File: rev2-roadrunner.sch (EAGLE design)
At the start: 22 parts, among them J1 USB_MINI-B_SMT, Y1 16MHz

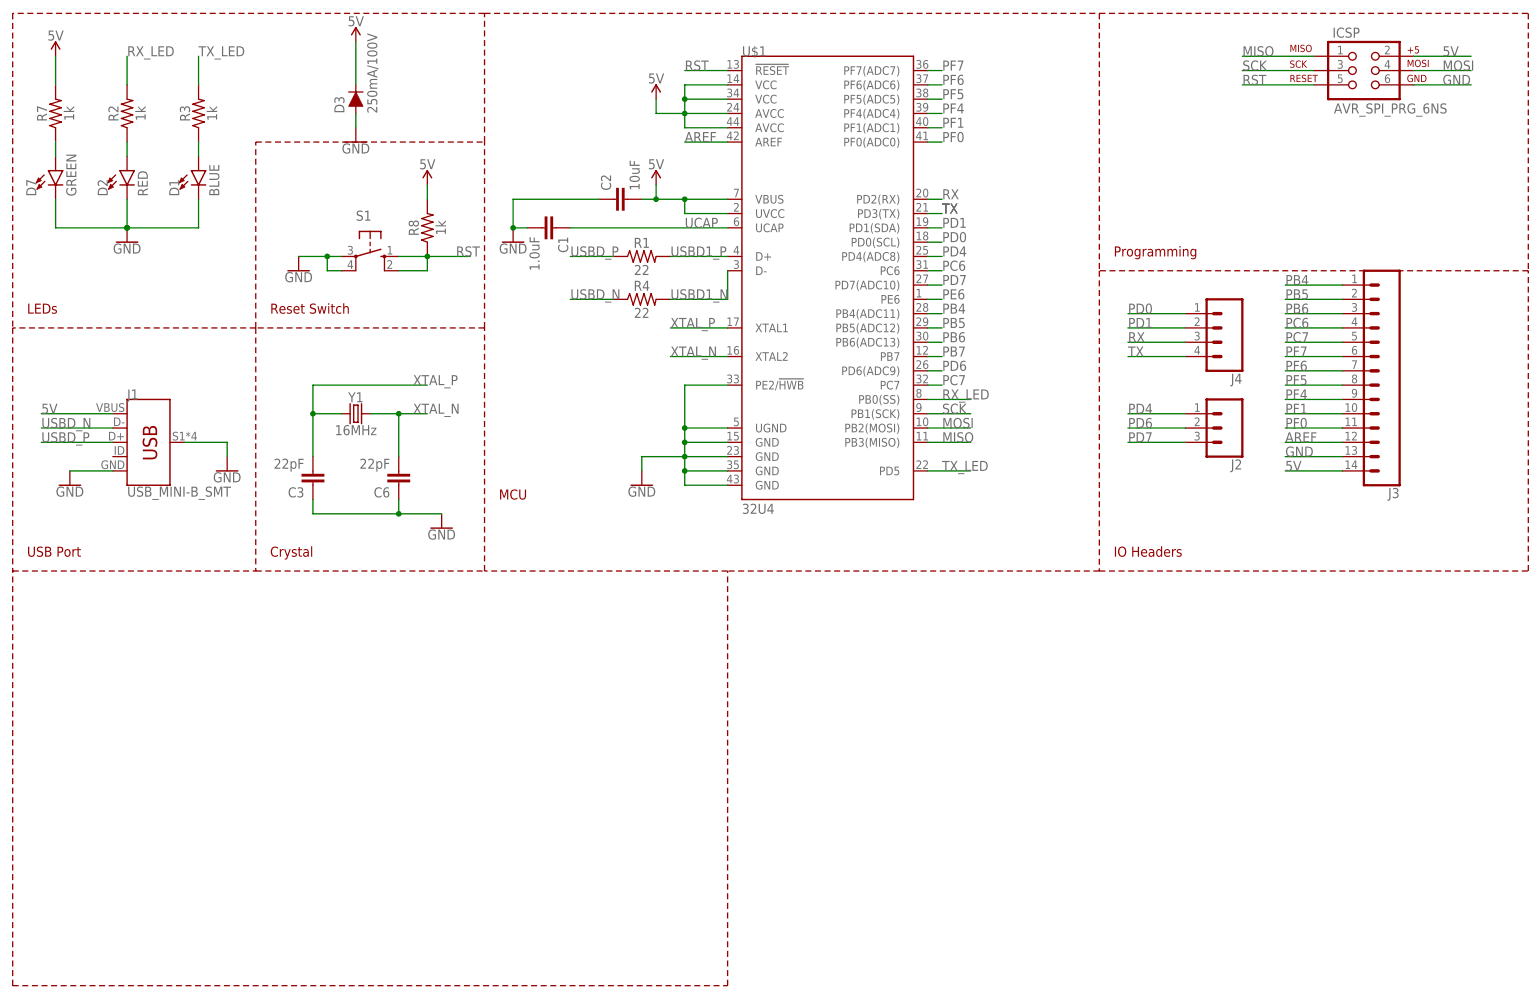
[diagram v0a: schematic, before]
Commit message: Finalized Board and Schematic design
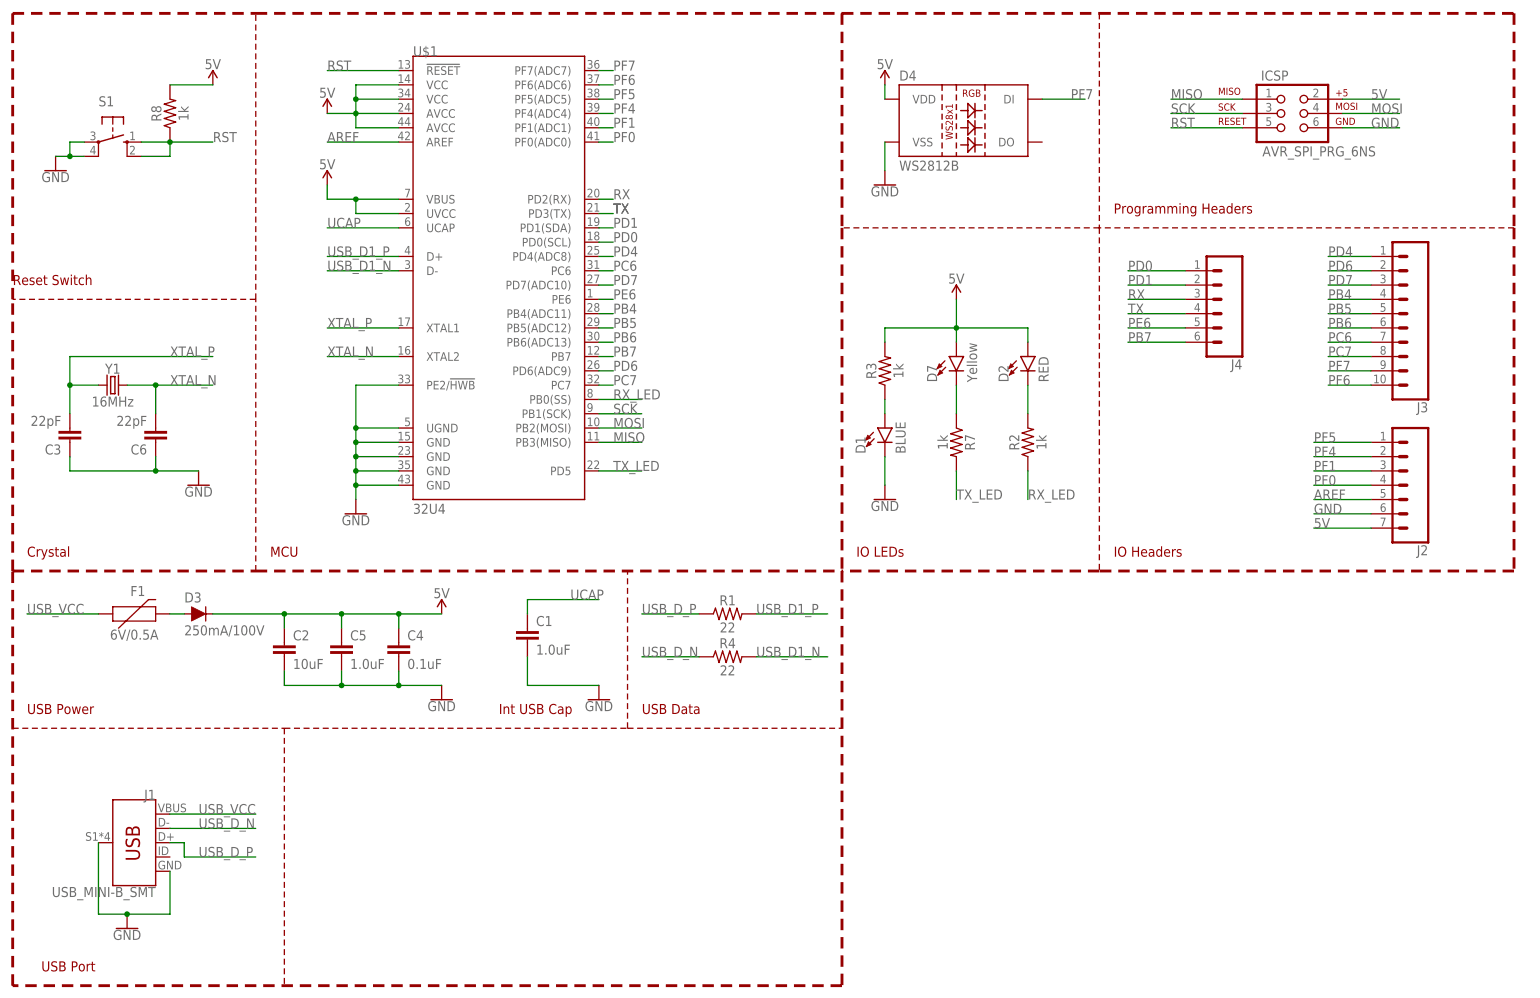
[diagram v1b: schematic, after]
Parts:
- added C4: 0.1uF, SparkFun-Capacitors:1.0UF-1206-50V-10%
- added C5: 1.0uF, SparkFun-Capacitors:1.0UF-1206-50V-10%
- added D4: WS2812B, SparkFun-LED:WS2812B
- added F1: 6V/0.5A, SparkFun-Fuses:PPTC_HALF-AMP
- D7: value GREEN -> Yellow; device SparkFun-LED:LED-GREEN1206 -> SparkFun-LED:LED-YELLOWLILYPAD
- J2: device SparkFun-Connectors:CONN_03 -> SparkFun-Connectors:CONN_07
- J3: device SparkFun-Connectors:CONN_14 -> SparkFun-Connectors:CONN_10"
- J4: device SparkFun-Connectors:CONN_04 -> SparkFun-Connectors:CONN_06SILK_FEMALE_PTH
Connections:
- net USBD1_N renamed USB_D1_N
- net USBD1_P renamed USB_D1_P
- net USBD_N renamed USB_D_N
- net USBD_P renamed USB_D_P
- new net N$4: D3.A, F1.2
- new net USB_VCC: F1.1, J1.VBUS
- net 5V: now also C2.1, C4.1, C5.1, D2.A, D4.VDD, D7.A, J2.7, R3.2; no longer C2.2, J1.VBUS, J3.14, R7.2
- net AREF: now also J2.5; no longer J3.12
- net GND: now also C2.2, C4.2, C5.2, D4.VSS, J2.6; no longer C2.1, D2.C, D3.A, D7.C, J3.13
- net N$2: now also D7.C, R7.1; no longer D2.A, R2.1
- net N$3: now also D2.C, R2.2; no longer D7.A, R7.1
- net PB4: now also J3.4; no longer J3.1
- net PB5: now also J3.5; no longer J3.2
- net PB6: now also J3.6; no longer J3.3
- net PB7: now also J4.6
- net PC6: now also J3.7; no longer J3.4
- net PC7: now also J3.8; no longer J3.5
- net PD4: now also J3.1; no longer J2.1
- net PD6: now also J3.2; no longer J2.2
- net PD7: now also J3.3; no longer J2.3
- net PE6: now also J4.5
- net PF0: now also J2.4; no longer J3.11
- net PF1: now also J2.3; no longer J3.10
- net PF4: now also J2.2; no longer J3.9
- net PF5: now also J2.1; no longer J3.8
- net PF6: now also J3.10; no longer J3.7
- net PF7: now also D4.DI, J3.9; no longer J3.6
- net RX_LED: now also R2.1; no longer R2.2
- net TX_LED: now also R7.2; no longer R3.2
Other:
- note added: "IO LEDs"
- note added: "Int USB Cap"
- note added: "Programming Headers"
- note added: "USB Data"
- note added: "USB Power"
- note removed: "LEDs"
- note removed: "Programming"
- moved on the sheet: C1, C2, C3, C6, D1, D2, D3, D7, ICSP, J1, R1, R2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
